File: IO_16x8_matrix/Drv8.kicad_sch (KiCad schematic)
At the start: 34 parts, among them J5 Conn_01x09, J6 Conn_01x09, Q1 MMBT3904, Q2 MMBT3904, Q3 MMBT3904, Q4 MMBT3904, Q5 MMBT3904, Q6 MMBT3904, Q7 MMBT3904, Q8 MMBT3904

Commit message: routed
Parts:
- J6: now in the parts list
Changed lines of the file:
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@@
   )
   (symbol (lib_id "Connector_Generic:Conn_01x09") (at 232.41 111.76 0) (unit 1)
-    (in_bom no) (on_board no) (fields_autoplaced)
+    (in_bom yes) (on_board yes) (fields_autoplaced)
     (property "Reference" "J6" (id 0) (at 234.95 110.4899 0)
       (effects (font (size 1.27 1.27)) (justify left))

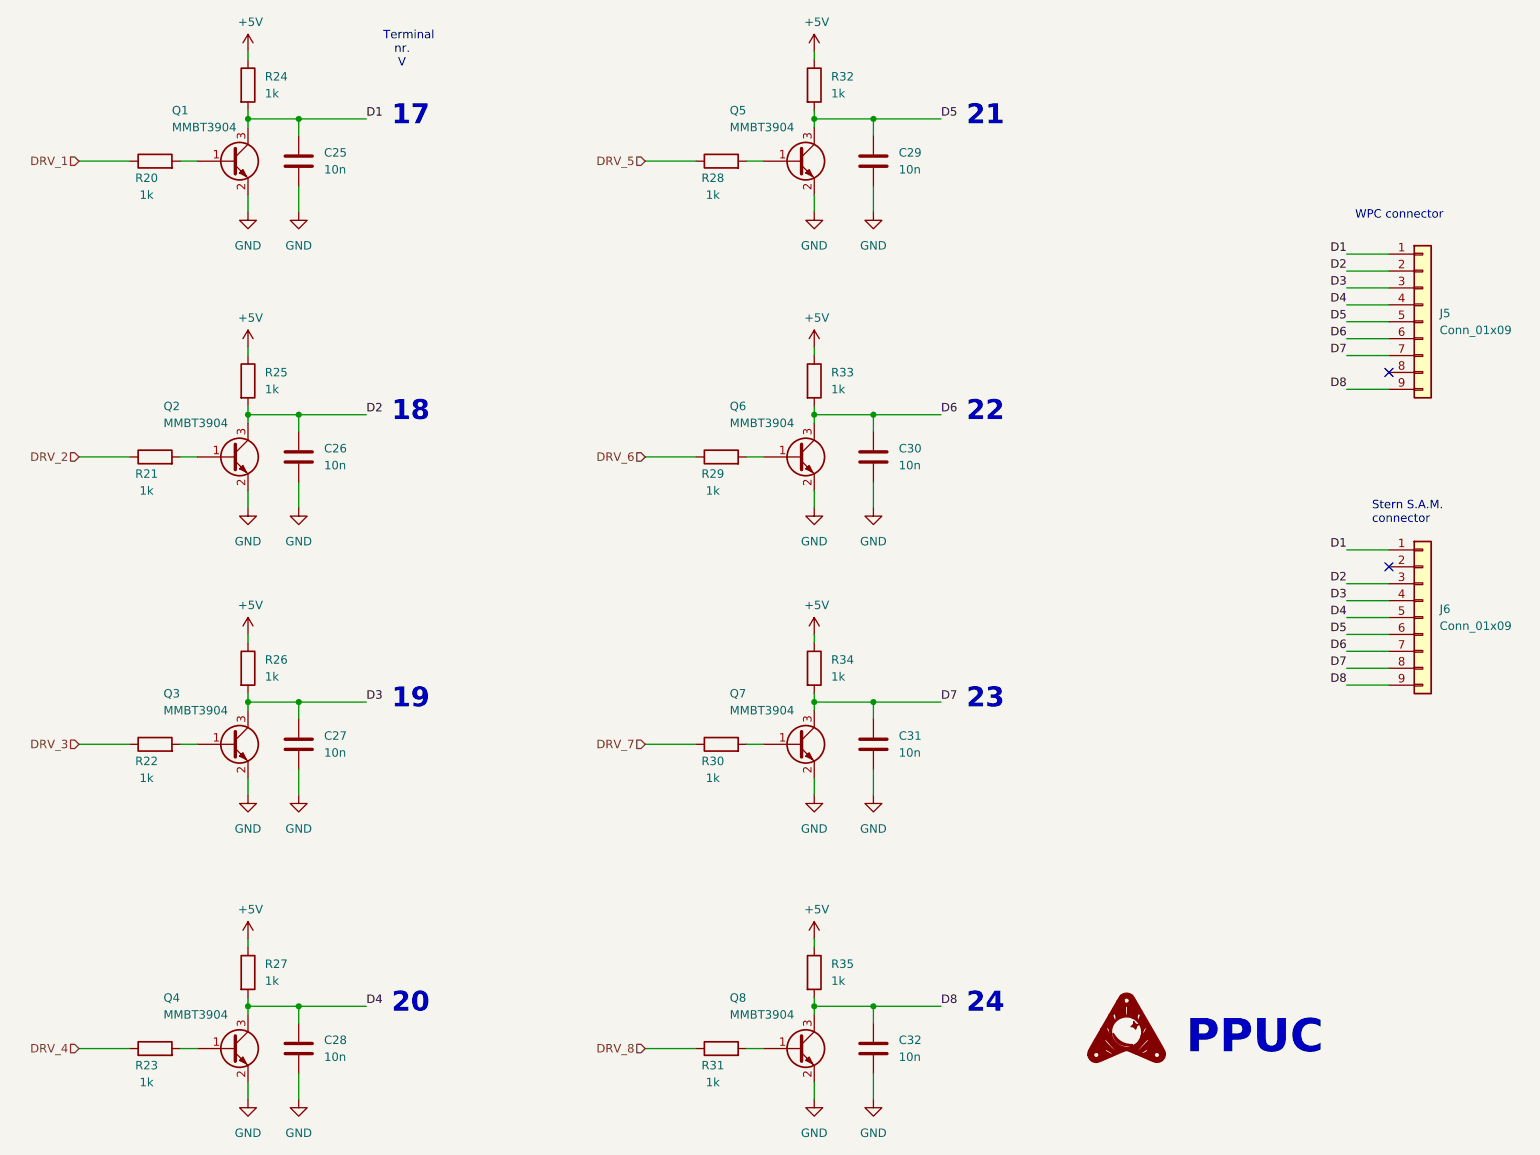
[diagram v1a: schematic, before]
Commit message: opt routing
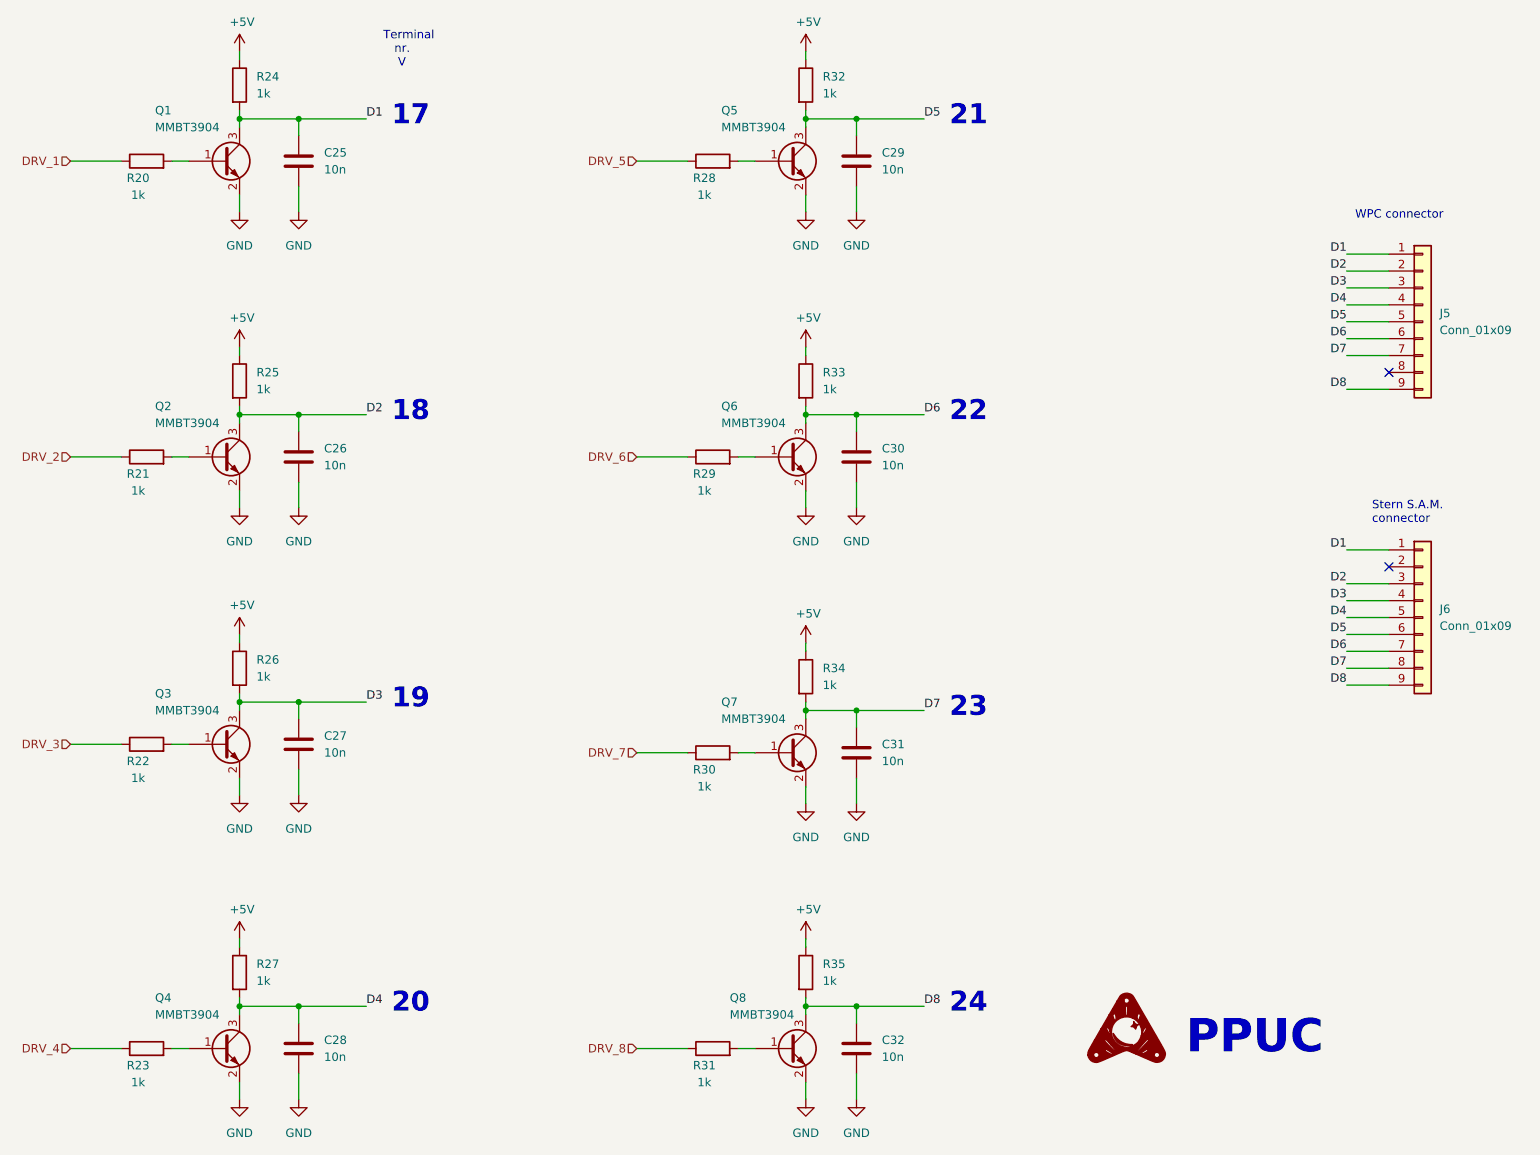
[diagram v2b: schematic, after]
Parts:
- J5: now left out of the parts list
- renumbered C32 to C25, C31 to C26, C30 to C27, C29 to C28, C28 to C29, C27 to C30, C26 to C31, C25 to C32, Q8 to Q1, Q7 to Q2, Q6 to Q3, Q5 to Q4, Q4 to Q5, Q3 to Q6, Q2 to Q7, Q1 to Q8, R31 to R20, R30 to R21, R29 to R22, R28 to R23, R35 to R24, R34 to R25, R33 to R26, R32 to R27, R23 to R28, R22 to R29, R21 to R30, R20 to R31, R27 to R32, R26 to R33, R25 to R34, R24 to R35
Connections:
- net D1: now also C25.1, Q1.3 (C), R24.2; no longer C32.1, Q8.3 (C), R35.2
- net D2: now also C26.1, Q2.3 (C), R25.2; no longer C31.1, Q7.3 (C), R34.2
- net D3: now also C27.1, Q3.3 (C), R26.2; no longer C30.1, Q6.3 (C), R33.2
- net D4: now also C28.1, Q4.3 (C), R27.2; no longer C29.1, Q5.3 (C), R32.2
- net D5: now also C29.1, Q5.3 (C), R32.2; no longer C28.1, Q4.3 (C), R27.2
- net D6: now also C30.1, Q6.3 (C), R33.2; no longer C27.1, Q3.3 (C), R26.2
- net D7: now also C31.1, Q7.3 (C), R34.2; no longer C26.1, Q2.3 (C), R25.2
- net D8: now also C32.1, Q8.3 (C), R35.2; no longer C25.1, Q1.3 (C), R24.2
- net DRV_1: now also R20.1; no longer R31.1
- net DRV_2: now also R21.1; no longer R30.1
- net DRV_3: now also R22.1; no longer R29.1
- net DRV_4: now also R23.1; no longer R28.1
- net DRV_5: now also R28.1; no longer R23.1
- net DRV_6: now also R29.1; no longer R22.1
- net DRV_7: now also R30.1; no longer R21.1
- net DRV_8: now also R31.1; no longer R20.1
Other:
- moved on the sheet: C25, C26, C27, C28, C29, C30, C31, C32, Q1, Q2, Q3, Q4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
